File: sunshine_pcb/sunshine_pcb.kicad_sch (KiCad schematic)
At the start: 17 parts, among them J1 XT30PW, J2 XT30PW, J3 MR30, J4 MR30, J5 USB_C_Receptacle_USB2.0_16P, SW1 Fingertech, U1 RP2350_60QFN, U2 W25Q128JVP, U3 LIS3MDL, U4 ADXL375, U5 HT7533, U6 FS2A, U7 DualAM32

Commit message: Do layout
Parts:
- removed J1, J2: XT30PW, Connector_AMASS:AMASS_XT30PW-M_1x02_P2.50mm_Horizontal, symbol custom:XT30PW
- added C10, C11, C13, C14, C15, C16, C17, C18, C19, C22, C25, C26, C27, C28, C30: 100nF, PCM_JLCPCB:C_0402, symbol PCM_JLCPCB-Capacitors:0402,100nF,(2)
- added C12, C29, C7, C8, C9: 4.7uF, PCM_JLCPCB:C_0402, symbol PCM_JLCPCB-Capacitors:0402,4.7uF
- added C23, C24: 15pF, PCM_JLCPCB:C_0402, symbol PCM_JLCPCB-Capacitors:0402,15pF
- added C3, C4: 10u, Capacitor_SMD:C_1210_3225Metric, symbol Device:C
- added C5, C6: 10uF, PCM_JLCPCB:C_0805, symbol PCM_JLCPCB-Capacitors:0805,10uF,(2)
- added D2, D3: 1N5819WS, PCM_JLCPCB:D_SOD-323, symbol PCM_JLCPCB-Diodes:Schottky,1N5819WS
- added D4, D5, D6: LED, LED_SMD:LED_PLCC_2835, symbol Device:LED
- added D7: SMF12A, PCM_JLCPCB:D_SOD-123FL, symbol PCM_JLCPCB-Diodes:TVS-Uni,SMF12A
- added J1, J2: Soldered, Connector_Wire:SolderWire-0.5sqmm_1x02_P4.6mm_D0.9mm_OD2.1mm_Relief, symbol Connector_Generic:Conn_01x02
- added Q1: AO3401A, PCM_JLCPCB:Q_SOT-23, symbol PCM_JLCPCB-Transistors:PMOS,AO3401A
- added R1, R15, R16, R17, R19, R2, R3: 5.1kΩ, PCM_JLCPCB:R_0402, symbol PCM_JLCPCB-Resistors:0402,5.1kΩ
- added R10, R12, R13, R14: 33Ω, PCM_JLCPCB:R_0805, symbol PCM_JLCPCB-Resistors:0805,33Ω
- added R11, R18, R7, R8, R9: 1kΩ, PCM_JLCPCB:R_0402, symbol PCM_JLCPCB-Resistors:0402,1kΩ
- added R4, R5, R6: 33Ω, PCM_JLCPCB:R_0402, symbol PCM_JLCPCB-Resistors:0402,33Ω
- added S1, S2: TS-1187A-C-B-B, PCM_JLCPCB:SW-SMD_4P-L5.1-W5.1-P3.70-LS6.5-TL-2, symbol PCM_JLCPCB-Connectors_Buttons:Tactile Button, 160gf, 12V, 50mA, 5.1mm
- added U8: USBLC6-2P6, Package_TO_SOT_SMD:SOT-666, symbol Power_Protection:USBLC6-2P6
- added Y1: ABM8-272-T3, Crystal:Crystal_SMD_3225-4Pin_3.2x2.5mm, symbol Device:Crystal_GND24
- J3, J4: value MR30 -> Soldered; footprint Connector_AMASS:AMASS_MR30PW-M_1x03_P3.50mm_Horizontal -> Connector_Wire:SolderWire-0.5sqmm_1x03_P4.6mm_D0.9mm_OD2.1mm_Relief; LCSC C19268036 -> C503478
- J5: value USB_C_Receptacle_USB2.0_16P -> VerticalUSB
- L1: value L -> 3.3u
- U1: footprint Package_DFN_QFN:QFN-60-1EP_7x7mm_P0.4mm_EP3.4x3.4mm -> Package_DFN_QFN:QFN-60-1EP_7x7mm_P0.4mm_EP3.4x3.4mm_ThermalVias
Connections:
- net GND: now also C1.2, C2.2, D1.1 (K), J5.A1 (GND), J5.A12 (GND), J5.B1 (GND), J5.B12 (GND), U1.47 (VREG_PGND), U1.61 (GND), U2.4 (GND), U2.9 (EP), U3.12 (GND), U3.2 (GND), U3.3 (GND), U4.2 (GND), U4.4 (GND), U4.5 (GND), U5.1 (GND), U6.6 (GND), C10.2, C11.2, C12.2, C13.2, C14.2, C15.2, C16.2, C17.2, C18.2, C19.2, C22.2, C23.1, C24.1, C25.2, C26.2, C27.2, C28.2, C29.2, C3.2, C30.2, C4.2, C5.2, C6.2, C7.2, C8.2, C9.2, D4.1 (K), D5.1 (K), D6.1 (K), D7.2, J2.2 (Pin_2), R1.2, R18.2, R2.2, R3.1, S1.3 (C), S1.4 (D), S2.3 (C), S2.4 (D), U8.2 (GND), Y1.2, Y1.4
- net S1: now also U1.9 (GPIO6)
- net S2: now also U1.12 (GPIO8)
- net VDC: now also C1.1, C2.1, SW1.2 (B), C3.1, C4.1, D7.1, R16.1
- net at U7.1 (M1A): now also J3.3 (Pin_3)
- net at U7.11 (+5V): now also D2.2
- net at U7.2 (M1B): now also J3.2 (Pin_2)
- net at U7.3 (M1C): now also J3.1 (Pin_1)
- net at U7.4 (M2A): now also J4.1 (Pin_1)
- net at U7.5 (M2B): now also J4.2 (Pin_2)
- net at U7.6 (M2C): now also J4.3 (Pin_3)
- net BATT1_+: now reaches SW1.1 (A)
- net BATT1_+: now also J1.1 (Pin_1)
- net VBUS: now reaches J5.A4 (VBUS), J5.A9 (VBUS), J5.B4 (VBUS), J5.B9 (VBUS)
- net VBUS: now also D3.2, U8.5 (VBUS)
- net at J5.A5 (CC1): now also R1.1
- net USB_C_D+: now reaches J5.A6 (D+)
- net USB_C_D+: now also J5.B6 (D+), U8.3 (I/O2)
- net USB_C_D-: now reaches J5.A7 (D-)
- net USB_C_D-: now also J5.B7 (D-), U8.1 (I/O1)
- net at J5.B5 (CC2): now also R2.1
- net at J5.S1 (SHIELD): now also R3.2
- net QSPI_SS: now reaches U2.1 (~{CS})
- net QSPI_SS: now also U1.60 (QSPI_SS), R7.1
- net QSPI_SD1: now reaches U2.2 (DO/IO_{1})
- net QSPI_SD1: now also U1.59 (QSPI_SD1)
- net QSPI_SD2: now reaches U2.3 (~{WP}/IO_{2})
- net QSPI_SD2: now also U1.58 (QSPI_SD2)
- net QSPI_SD0: now reaches U2.5 (DI/IO_{0})
- net QSPI_SD0: now also U1.57 (QSPI_SD0)
- net QSPI_SCK: now reaches U2.6 (CLK)
- net QSPI_SCK: now also U1.56 (QSPI_SCLK)
- net QSPI_SD3: now reaches U2.7 (~{HOLD}/~{RESET}/IO_{3})
- net QSPI_SD3: now also U1.55 (QSPI_SD3)
- net +3V3: now reaches U2.8 (VCC)
- net +3V3: now also U1.1 (IOVDD), U1.11 (IOVDD), U1.20 (IOVDD), U1.30 (IOVDD), U1.38 (IOVDD), U1.44 (ADC_AVDD), U1.45 (IOVDD), U1.49 (VREG_VIN), U1.53 (USB_OTP_VDD), U1.54 (QSPI_IOVDD), U3.5 (Vdd), U3.6 (Vdd_IO), U4.1 (Vdd_I/O), U4.6 (Vs), U5.3 (VOUT), C13.1, C14.1, C15.1, C16.1, C17.1, C18.1, C19.1, C22.1, C25.1, C26.1, C28.1, C29.1, C6.1, C8.1, R4.1
- net at D1.2 (A): now also R10.2
- net +5V: now reaches U5.2 (VIN)
- net +5V: now also U6.5 (+5V), C5.1, D2.1, D3.1, Q1.2 (S), R19.1
- net IMU_MISO: now reaches U4.12 (SDO/ADDR)
- net IMU_MISO: now also U1.16 (GPIO12)
- net IMU_MOSI: now reaches U4.13 (SDA/SDI/SDIO)
- net IMU_MOSI: now also U1.15 (GPIO11)
- net IMU_SCK: now reaches U4.14 (SCL/SCLK)
- net IMU_SCK: now also U1.14 (GPIO10)
- net IMU_CS: now reaches U4.7 (~{CS})
- net IMU_CS: now also U1.17 (GPIO13)
- net IMU_INT1: now reaches U4.8 (INT1)
- net IMU_INT1: now also U1.18 (GPIO14)
- net IMU_INT2: now reaches U4.9 (INT2)
- net IMU_INT2: now also U1.19 (GPIO15)
- net R1: now reaches U6.1
- net R1: now also U1.3 (GPIO1)
- net R2: now reaches U6.2
- net R2: now also U1.5 (GPIO3)
- net R3: now reaches U6.3
- net R3: now also U1.8 (GPIO5)
- net R4: now reaches U6.4
- net R4: now also U1.10 (GPIO7)
- net +1V1: now reaches L1.1
- net +1V1: now also U1.23 (DVDD), U1.39 (DVDD), U1.50 (VREG_FB), U1.6 (DVDD), C10.1, C11.1, C12.1, C9.1
- net VREG_LX: now reaches L1.2
- net VREG_LX: now also U1.48 (VREG_LX)
- net LED: now reaches U1.13 (GPIO9)
- net LED: now also R11.1
- net at U1.21 (XIN): now also C23.2, Y1.3
- net at U1.22 (XOUT): now also R8.2
- net RESET: now reaches U1.26 (RUN)
- net RESET: now also R9.1
- net MAG_MISO: now reaches U1.27 (GPIO16)
- net MAG_MISO: now also U3.9 (SDO/SA1)
- net MAG_CS: now reaches U1.28 (GPIO17)
- net MAG_CS: now also U3.10 (~{CS})
- net MAG_SCK: now reaches U1.29 (GPIO18)
- net MAG_SCK: now also U3.1 (SCL/SPC)
- net MAG_MOSI: now reaches U1.31 (GPIO19)
- net MAG_MOSI: now also U3.11 (SDA/SDI/SDO)
- net MAG_DRDY: now reaches U1.32 (GPIO20)
- net MAG_DRDY: now also U3.8 (DRDY)
- net MAG_INT: now reaches U1.33 (GPIO21)
- net MAG_INT: now also U3.7 (INT)
- net at U1.40 (GPIO26_ADC0): now also C30.1, R15.2, R17.1
- net VREG_AVDD: now reaches U1.46 (VREG_AVDD)
- net VREG_AVDD: now also C7.1, R4.2
- net at U1.51 (USB_DM): now also R6.1
- net at U1.52 (USB_DP): now also R5.1
- net at U3.4 (C1): now also C27.1
- new net: R15.1, R16.2
- new net: C24.2, R8.1, Y1.1
- new net: Q1.3 (D), R10.1, R12.1, R13.1, R14.1
- new net: D6.2 (A), R14.2
- new net: Q1.1 (G), R11.2, R19.2
- new net: D4.2 (A), R12.2
- new net: R9.2, S2.1 (A), S2.2 (B)
- new net: R17.2, R18.1
- new net: R7.2, S1.1 (A), S1.2 (B)
- new net: D5.2 (A), R13.2
- new net BATT2_+: J1.2 (Pin_2), J2.1 (Pin_1)
- new net USB_D+: R5.2, U8.4 (I/O2)
- new net USB_D-: R6.2, U8.6 (I/O1)
- no-connect marks 0 -> 16
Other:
- moved on the sheet: C1, C2, D1, J3, J4, J5, L1, SW1, U1, U2, U3, U4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

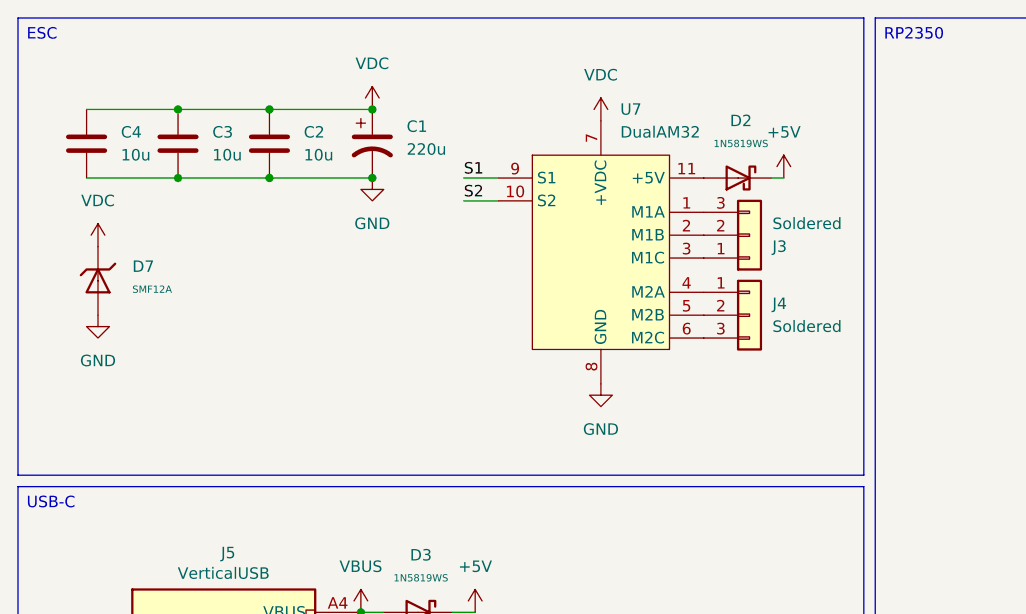
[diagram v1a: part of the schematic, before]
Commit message: Add some protection
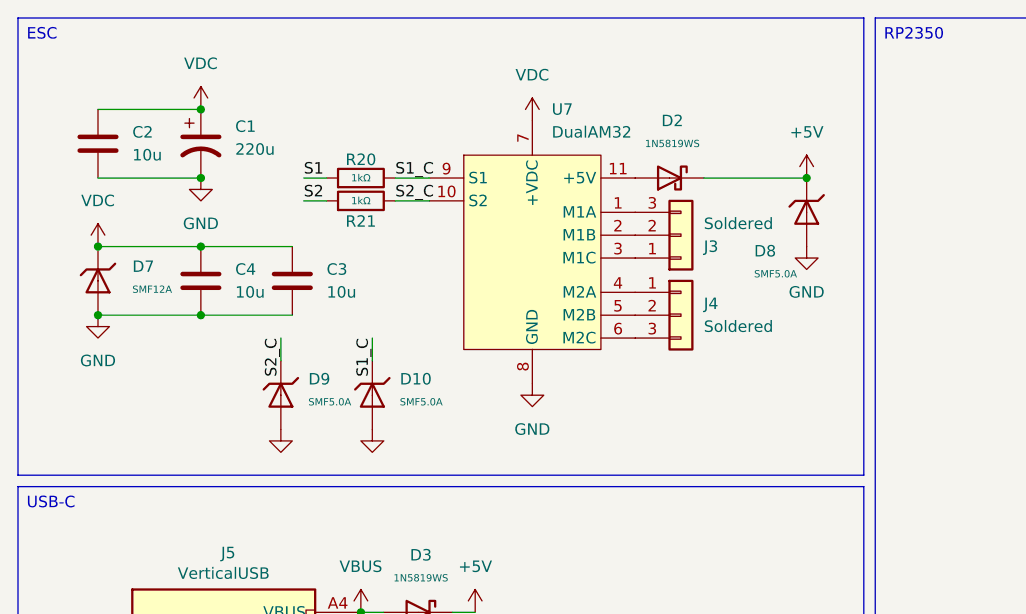
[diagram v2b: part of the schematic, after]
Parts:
- added D10, D8, D9: SMF5.0A, PCM_JLCPCB:D_SOD-123FL, symbol PCM_JLCPCB-Diodes:TVS-Uni,SMF5.0A
- added R20, R21: 1kΩ, PCM_JLCPCB:R_0402, symbol PCM_JLCPCB-Resistors:0402,1kΩ
- J1, J2: footprint Connector_Wire:SolderWire-0.5sqmm_1x02_P4.6mm_D0.9mm_OD2.1mm_Relief -> Connector_Wire:SolderWire-0.75sqmm_1x02_P4.8mm_D1.25mm_OD2.3mm_Relief
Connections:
- net +5V: now also D8.1
- net GND: now also D10.2, D8.2, D9.2
- net S1: now also R20.1; no longer U7.9 (S1)
- net S2: now also R21.1; no longer U7.10 (S2)
- new net S1_C: D10.1, R20.2, U7.9 (S1)
- new net S2_C: D9.1, R21.2, U7.10 (S2)
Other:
- moved on the sheet: C1, C2, C3, C4, D2, J3, J4, U7
